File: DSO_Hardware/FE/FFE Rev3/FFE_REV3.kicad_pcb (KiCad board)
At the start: 4 copper layers, 43.2 x 41.4 mm, 87 parts, among them J1 BNC, J2 SMA, J3 Conn_02x07_Odd_Even, K1 FTR-B3GA, K2 FTR-B3GA, Q1 DMN62D0UW, Q2 DMN62D0UW, Q3 Q_NJFET_DSG, Q4 Q_NPN_BEC, U1 CPC1017, U2 TBD, U3 OP07, U4 LM27761

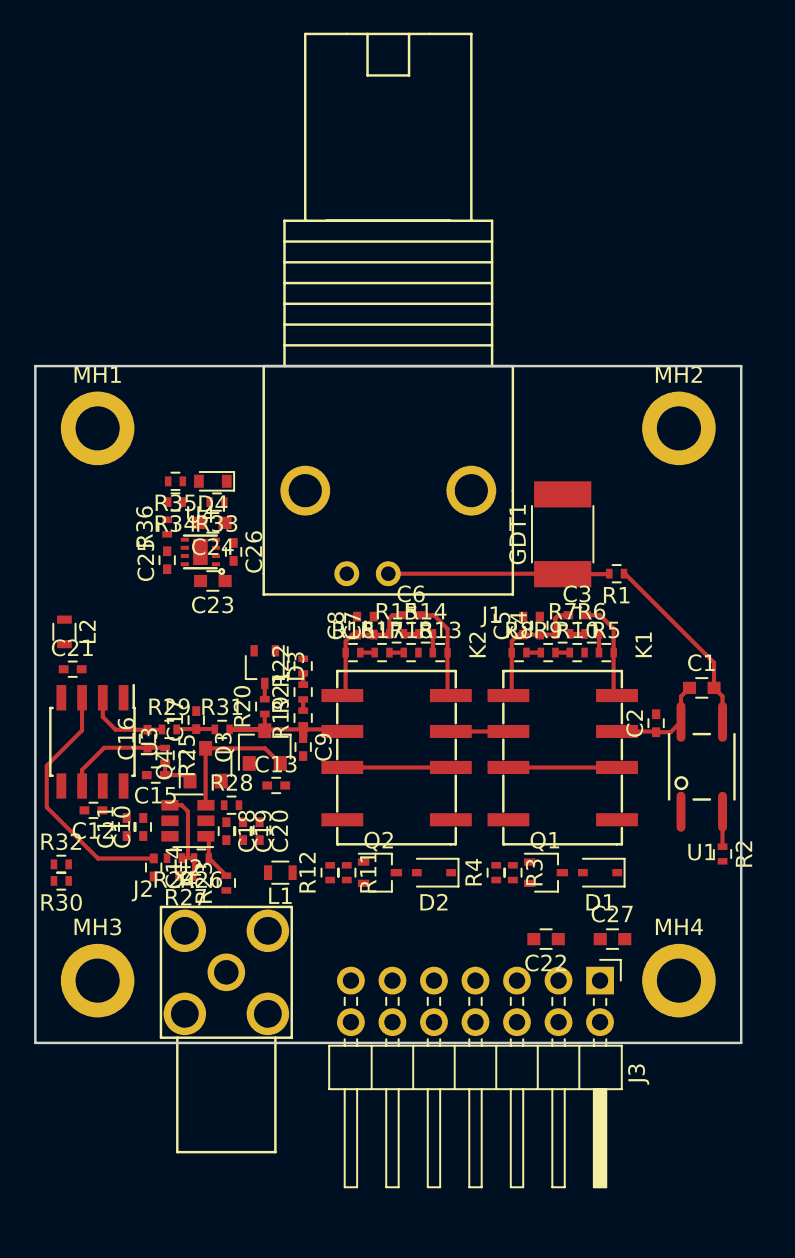
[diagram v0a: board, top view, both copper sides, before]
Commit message: FFE Rev3 Done
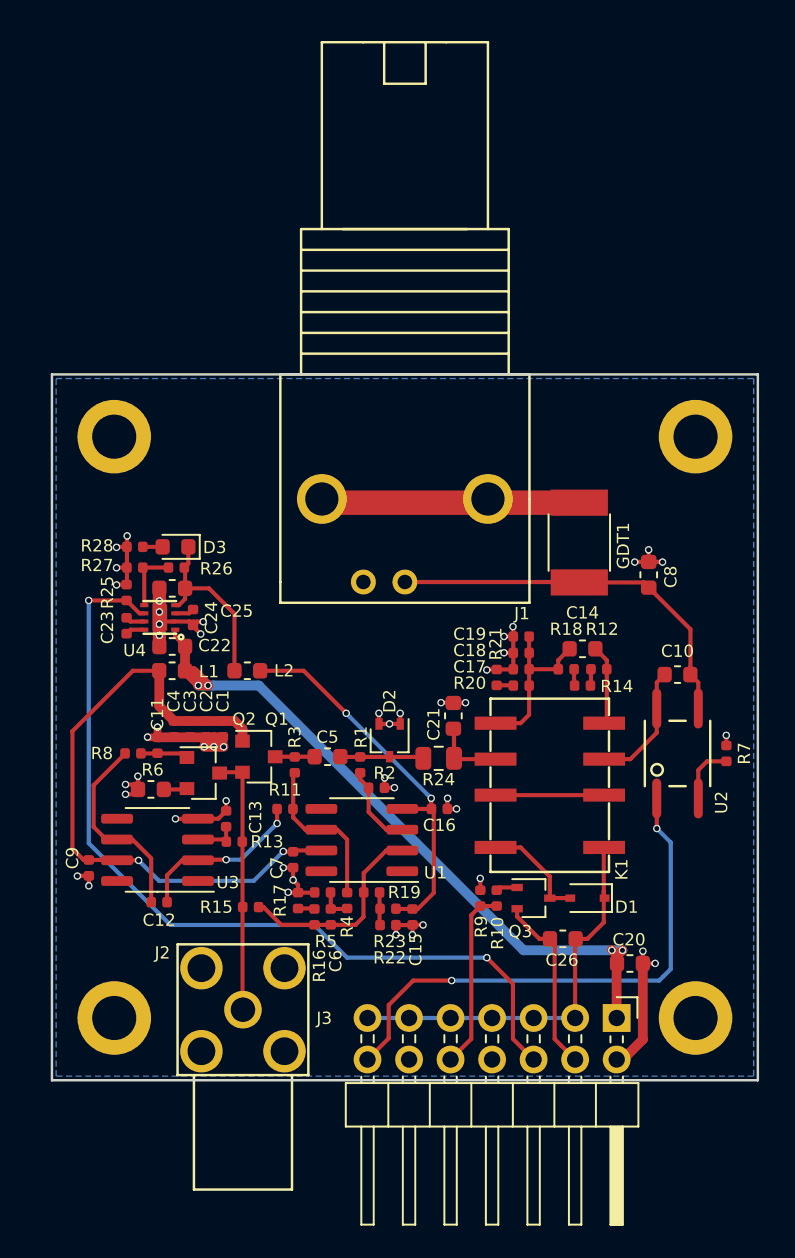
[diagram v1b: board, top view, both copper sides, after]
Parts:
- removed the C20 at (124.5, 91.4)
- removed the C21 at (113.0, 81.5)
- removed the C3 at (143.9, 78.2)
- removed the C7 at (131.4, 78.9)
- removed the C8 at (130.4, 78.9)
- removed the D2 at (135.1, 94.0)
- removed K2: FTR-B3GA, DSO:FTR-B3G
- removed the Q1 at (142.0, 94.0)
- removed the Q2 at (131.8, 94.0)
- removed the R11 at (129.8, 94.0)
- removed the R13 at (135.5, 80.5)
- removed the R26 at (120.9, 93.1)
- removed the R27 at (120.0, 94.2)
- removed R30, R32: 10k, Resistors_SMD:R_0402
- removed R31: 10M, Resistors_SMD:R_0402
- removed the R6 at (144.8, 79.4)
- removed the R7 at (143.0, 79.4)
- removed the R8 at (140.3, 80.5)
- removed the U2 at (120.1, 90.8)
- added C1: 100p, Capacitor_SMD:C_0402_1005Metric, F.Cu at (122.2, 85.2)
- added C14: 8p, Capacitor_SMD:C_0603_1608Metric, F.Cu at (144.2, 80.3)
- added C15: 0.1uF, Capacitor_SMD:C_0402_1005Metric, F.Cu at (133.8, 96.7)
- added C9: 0.1uF, Capacitor_SMD:C_0402_1005Metric, F.Cu at (114.0, 93.7)
- added Q3: DMN62D0UW, Package_TO_SOT_SMD:SOT-323_SC-70, F.Cu at (141.2, 95.5)
- added R2: 100K, Resistor_SMD:R_0402_1005Metric, F.Cu at (131.6, 88.8)
- added R24: 100, Resistor_SMD:R_0805_2012Metric, F.Cu at (135.4, 87.0)
- added U1: OP07, Package_SO:SOIC-8_3.9x4.9mm_P1.27mm, F.Cu at (130.7, 92.0)
- C10: renamed from C1; footprint Capacitors_SMD:C_0603 -> Capacitor_SMD:C_0603_1608Metric
- C11: renamed from C15; value 300pF -> 330p; footprint Capacitors_SMD:C_0402 -> Capacitor_SMD:C_0402_1005Metric
- C12: value 1n -> 1u; footprint Capacitors_SMD:C_0402 -> Capacitor_SMD:C_0402_1005Metric
- C13: renamed from C14; value 0.1uF -> 1u; footprint Capacitors_SMD:C_0402 -> Capacitor_SMD:C_0402_1005Metric
- C16: value 10nF -> 0.1uF; footprint Capacitors_SMD:C_0402 -> Capacitor_SMD:C_0402_1005Metric
- C17: value 0.1uF -> 390p; footprint Capacitors_SMD:C_0402 -> Capacitor_SMD:C_0402_1005Metric
- C18: value 1n -> 390p; footprint Capacitors_SMD:C_0402 -> Capacitor_SMD:C_0402_1005Metric
- C19: value 0.1uF -> DNP; footprint Capacitors_SMD:C_0402 -> Capacitor_SMD:C_0402_1005Metric
- C2: renamed from C10; footprint Capacitors_SMD:C_0402 -> Capacitor_SMD:C_0402_1005Metric
- C20: renamed from C27; footprint Capacitors_SMD:C_0603 -> Capacitor_SMD:C_0603_1608Metric
- C21: renamed from C9; value 6pF -> 3p; footprint Capacitors_SMD:C_0402 -> Capacitor_SMD:C_0603_1608Metric
- C22: renamed from C23; footprint Capacitors_SMD:C_0603 -> Capacitor_SMD:C_0603_1608Metric
- C23: renamed from C25; footprint Capacitors_SMD:C_0402 -> Capacitor_SMD:C_0402_1005Metric
- C24: renamed from C26; footprint Capacitors_SMD:C_0402 -> Capacitor_SMD:C_0402_1005Metric
- C25: renamed from C24; footprint Capacitors_SMD:C_0603 -> Capacitor_SMD:C_0603_1608Metric
- C26: renamed from C22; footprint Capacitors_SMD:C_0603 -> Capacitor_SMD:C_0603_1608Metric
- C3: renamed from C11; value 0.1uF -> 10n; footprint Capacitors_SMD:C_0402 -> Capacitor_SMD:C_0402_1005Metric
- C4: value 47pF -> 100n; footprint Capacitors_SMD:C_0402 -> Capacitor_SMD:C_0402_1005Metric
- C5: value 33pF -> 22n; footprint Capacitors_SMD:C_0402 -> Capacitor_SMD:C_0603_1608Metric
- C6: value 10pF -> 100n; footprint Capacitors_SMD:C_0402 -> Capacitor_SMD:C_0402_1005Metric
- C7: renamed from C13; footprint Capacitors_SMD:C_0402 -> Capacitor_SMD:C_0402_1005Metric
- C8: renamed from C2; footprint Capacitors_SMD:C_0402 -> Capacitor_SMD:C_0603_1608Metric
- D1: footprint Diodes_SMD:D_SOD-323 -> Diode_SMD:D_SOD-323
- D3: renamed from D4; footprint Diodes_SMD:D_0603 -> Diode_SMD:D_0603_1608Metric
- L1, L2: footprint Resistors_SMD:R_0603 -> Resistor_SMD:R_0603_1608Metric
- Q1: renamed from Q3; value Q_NJFET_DSG -> CPH3910
- Q2: renamed from Q4; value Q_NPN_BEC -> 2N3904
- R1: value 15 -> 900K; footprint Resistors_SMD:R_0402 -> Resistor_SMD:R_0402_1005Metric
- R10: value 33.2k -> 1k; footprint Resistors_SMD:R_0402 -> Resistor_SMD:R_0402_1005Metric
- R11: renamed from R29; value 10k -> 1M; footprint Resistors_SMD:R_0402 -> Resistor_SMD:R_0402_1005Metric
- R12: value 10k -> 330k; footprint Resistors_SMD:R_0402 -> Resistor_SMD:R_0402_1005Metric
- R13: renamed from R24; value 10M -> 1M; footprint Resistors_SMD:R_0402 -> Resistor_SMD:R_0402_1005Metric
- R14: value 300k -> 330k; footprint Resistors_SMD:R_0402 -> Resistor_SMD:R_0402_1005Metric
- R15: value 300k -> 900K; footprint Resistors_SMD:R_0402 -> Resistor_SMD:R_0402_1005Metric
- R16: value 39k -> 100K; footprint Resistors_SMD:R_0402 -> Resistor_SMD:R_0402_1005Metric
- R17: value 39k -> 15k; footprint Resistors_SMD:R_0402 -> Resistor_SMD:R_0402_1005Metric
- R18: value 33.2k -> 330k; footprint Resistors_SMD:R_0402 -> Resistor_SMD:R_0402_1005Metric
- R19: value 332k -> 900K; footprint Resistors_SMD:R_0402 -> Resistor_SMD:R_0402_1005Metric
- R20: value 3.3k -> 100; footprint Resistors_SMD:R_0402 -> Resistor_SMD:R_0402_1005Metric
- R21: value 390k -> 10k; footprint Resistors_SMD:R_0402 -> Resistor_SMD:R_0402_1005Metric
- R22: value 390k -> 1k; footprint Resistors_SMD:R_0402 -> Resistor_SMD:R_0402_1005Metric
- R23: value 50 -> 1k; footprint Resistors_SMD:R_0402 -> Resistor_SMD:R_0402_1005Metric
- R25: renamed from R36; footprint Resistors_SMD:R_0402 -> Resistor_SMD:R_0402_1005Metric
- R26: renamed from R33; footprint Resistors_SMD:R_0402 -> Resistor_SMD:R_0402_1005Metric
- R27: renamed from R34; footprint Resistors_SMD:R_0402 -> Resistor_SMD:R_0402_1005Metric
- R28: renamed from R35; footprint Resistors_SMD:R_0402 -> Resistor_SMD:R_0402_1005Metric
- R3: value 1k -> 1M; footprint Resistors_SMD:R_0402 -> Resistor_SMD:R_0402_1005Metric
- R4: value 10k -> 900K; footprint Resistors_SMD:R_0402 -> Resistor_SMD:R_0402_1005Metric
- R5: value 300k -> 100K; footprint Resistors_SMD:R_0402 -> Resistor_SMD:R_0402_1005Metric
- R6: renamed from R28; footprint Resistors_SMD:R_0402 -> Resistor_SMD:R_0603_1608Metric
- R7: renamed from R2; footprint Resistors_SMD:R_0402 -> Resistor_SMD:R_0402_1005Metric
- R8: renamed from R25; footprint Resistors_SMD:R_0402 -> Resistor_SMD:R_0402_1005Metric
- R9: value 39k -> 10k; footprint Resistors_SMD:R_0402 -> Resistor_SMD:R_0402_1005Metric
- U2: renamed from U1; value CPC1017 -> CPC1014
- U3: footprint Housings_SOIC:SOIC-8_3.9x4.9mm_Pitch1.27mm -> Package_SO:SOIC-8_3.9x4.9mm_P1.27mm
- moved C4 23.3 mm to (119.2, 85.2), turned to 270 degrees
- moved R5 22.7 mm to (128.3, 95.2), turned to 180 degrees
- moved C18 21.1 mm to (140.5, 80.5), turned to 180 degrees
- moved C19 20.8 mm to (140.5, 79.5), turned to 180 degrees
- moved R12 20.6 mm to (145.2, 81.5), turned to 0 degrees
- moved C17 20.1 mm to (140.5, 81.5), turned to 180 degrees
- moved R1 19.6 mm to (130.6, 87.4), turned to 270 degrees
- moved C6 19.1 mm to (128.8, 96.7), turned to 90 degrees
- moved R15 18.9 mm to (123.9, 96.1)
- moved C16 18.4 mm to (135.5, 90.1), turned to 0 degrees
- moved R22 16.7 mm to (132.3, 97.2), turned to 180 degrees
- moved R16 16.3 mm to (127.8, 96.7), turned to 90 degrees
- moved R17 16.0 mm to (126.8, 95.7), turned to 90 degrees
- moved R10 15.8 mm to (139.0, 95.5), turned to 270 degrees
- moved R20 15.7 mm to (140.5, 82.5), turned to 180 degrees
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- renumbered D3 to D2
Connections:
- C10 pad 1: /Attenuators/IN -> Net-(C10-Pad1)
- C10 pad 2: Net-(C1-Pad2) -> Net-(C10-Pad2)
- C12 pad 1: VDD -> Net-(C12-Pad1)
- C12 pad 2: GND -> Net-(C12-Pad2)
- C16 pad 1: Net-(C16-Pad1) -> VSS
- C16 pad 2: Net-(C16-Pad2) -> GND
- C17 pad 1: Net-(C17-Pad1) -> Net-(C14-Pad1)
- C18 pad 1: VSS -> Net-(C14-Pad1)
- C19 pad 1: VSS -> Net-(C14-Pad1)
- C21 pad 1: /BUFFER -> Net-(C21-Pad1)
- C4 pad 1: Net-(C3-Pad1) -> VDD
- C5 pad 1: Net-(C3-Pad1) -> Net-(C5-Pad1)
- C5 pad 2: GND -> /BUFFER
- C8 pad 1: /Attenuators/IN -> Net-(C10-Pad2)
- D2 pad 3: Net-(D3-Pad3) -> /BUFFER
- GDT1 pad 1: Net-(GDT1-Pad1) -> Net-(C10-Pad2)
- J1 pad 1: Net-(GDT1-Pad1) -> Net-(C10-Pad2)
- J3 pad 10: /-20dB_EN_2 -> /-40dB_EN
- J3 pad 8: /-20dB_EN_1 -> (no net)
- K1 pad 3: /Attenuators/IN -> Net-(C10-Pad1)
- K1 pad 4: Net-(C3-Pad2) -> Net-(C14-Pad2)
- K1 pad 5: Net-(C3-Pad1) -> Net-(C14-Pad1)
- K1 pad 6: Net-(K1-Pad6) -> Net-(C21-Pad1)
- Q1 pad 2: Net-(Q3-Pad2) -> Net-(J2-Pad1)
- Q1 pad 3: /BUFFER -> Net-(C5-Pad1)
- Q2 pad 3: Net-(Q3-Pad2) -> Net-(J2-Pad1)
- R1 pad 1: Net-(C1-Pad2) -> /BUFFER
- R1 pad 2: Net-(GDT1-Pad1) -> Net-(R1-Pad2)
- R10 pad 1: Net-(R10-Pad1) -> Net-(Q3-Pad1)
- R10 pad 2: GND -> /-40dB_EN
- R11 pad 1: Net-(C16-Pad2) -> Net-(C12-Pad2)
- R11 pad 2: Net-(C17-Pad1) -> Net-(R11-Pad2)
- R12 pad 1: /-20dB_EN_2 -> Net-(R12-Pad1)
- R12 pad 2: GND -> Net-(C14-Pad2)
- R13 pad 1: Net-(R24-Pad1) -> Net-(J2-Pad1)
- R14 pad 2: Net-(R13-Pad1) -> Net-(R12-Pad1)
- R15 pad 1: Net-(C6-Pad1) -> Net-(J2-Pad1)
- R15 pad 2: Net-(R14-Pad1) -> Net-(C6-Pad1)
- R17 pad 2: Net-(R17-Pad2) -> GND
- R18 pad 1: Net-(R17-Pad2) -> Net-(C14-Pad1)
- R18 pad 2: GND -> Net-(R14-Pad1)
- R19 pad 1: /BUFFER -> Net-(R19-Pad1)
- R19 pad 2: Net-(R19-Pad2) -> Net-(C6-Pad1)
- R20 pad 1: /BUFFER -> Net-(C14-Pad1)
- R20 pad 2: Net-(D3-Pad3) -> Net-(R20-Pad2)
- R21 pad 1: Net-(R19-Pad2) -> Net-(R20-Pad2)
- R21 pad 2: Net-(R21-Pad2) -> GND
- R22 pad 1: Net-(R21-Pad2) -> GND
- R22 pad 2: GND -> Net-(R19-Pad1)
- R23 pad 1: Net-(J2-Pad1) -> Net-(R19-Pad1)
- R23 pad 2: Net-(R23-Pad2) -> VSS
- R3 pad 1: Net-(Q1-Pad1) -> Net-(C5-Pad1)
- R3 pad 2: /-20dB_EN_1 -> Net-(R11-Pad2)
- R4 pad 1: /-20dB_EN_1 -> Net-(R11-Pad2)
- R4 pad 2: GND -> Net-(C6-Pad2)
- R5 pad 1: Net-(R5-Pad1) -> Net-(C6-Pad2)
- R5 pad 2: Net-(C3-Pad2) -> GND
- R6 pad 2: VSS -> GND
- R8 pad 1: Net-(C16-Pad1) -> Net-(C12-Pad1)
- R9 pad 1: Net-(R8-Pad2) -> /-40dB_EN
- R9 pad 2: Net-(R10-Pad1) -> GND
- U2 pad 3: Net-(C1-Pad2) -> Net-(C10-Pad2)
- U2 pad 4: /Attenuators/IN -> Net-(C10-Pad1)
- U3 pad 2: Net-(C16-Pad2) -> Net-(C12-Pad2)
- U3 pad 4: VSS -> GND
- U3 pad 6: Net-(C16-Pad1) -> Net-(C12-Pad1)
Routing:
- net GND: track 0.00 -> 89.1 mm, vias 0 -> 48
- net /CHANNEL_EN: track 0.00 -> 53.2 mm, vias 0 -> 2
- net +5VA: track 0.00 -> 43.9 mm, vias 0 -> 4
- net VDD: track 0.00 -> 39.5 mm, vias 0 -> 2
- net /DC_CPL_EN: track 0.00 -> 32.8 mm, vias 0 -> 2
- net +VUSB: track 0.00 -> 24.7 mm
- net VSS: track 0.00 -> 24.2 mm, vias 0 -> 2
- net Net-(C10-Pad2): track 0.00 -> 23.7 mm
- net Net-(J2-Pad1): track 0.00 -> 16.0 mm
- net Net-(GDT1-Pad1): track 13.5 -> 0.00 mm
- net Net-(C13-Pad1): track 15.4 -> 2.71 mm
- net Net-(C12-Pad1): track 0.00 -> 12.3 mm
- net Net-(C1-Pad2): track 11.6 -> 0.00 mm
- net -5VA: track 0.00 -> 11.2 mm
- net /-40dB_EN: track 0.00 -> 11.1 mm
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- added copper zone on B.Cu, net GND
- added copper zone on In1.Cu, net GND
- added copper zone on In2.Cu, net GND
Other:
- board size 43.2 x 41.4 mm -> 43.2 x 43.2 mm
- net class Default: via_dia 0.6 -> 0.4572; via_drill 0.4 -> 0.3
- rule trace_min: 0.2 -> 0.254
- rule via_min_drill: 0.3 -> 0.254
- rule via_min_size: 0.4 -> 0.4572
